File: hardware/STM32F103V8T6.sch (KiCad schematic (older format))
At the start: 34 parts, among them J14 STM32_USB_DEBUG, J15 STM32_GTR, J16 SPI_DEBUG, J17 SWD, SW2 RST, U6 STM32F407VET6, Y3 O_8M

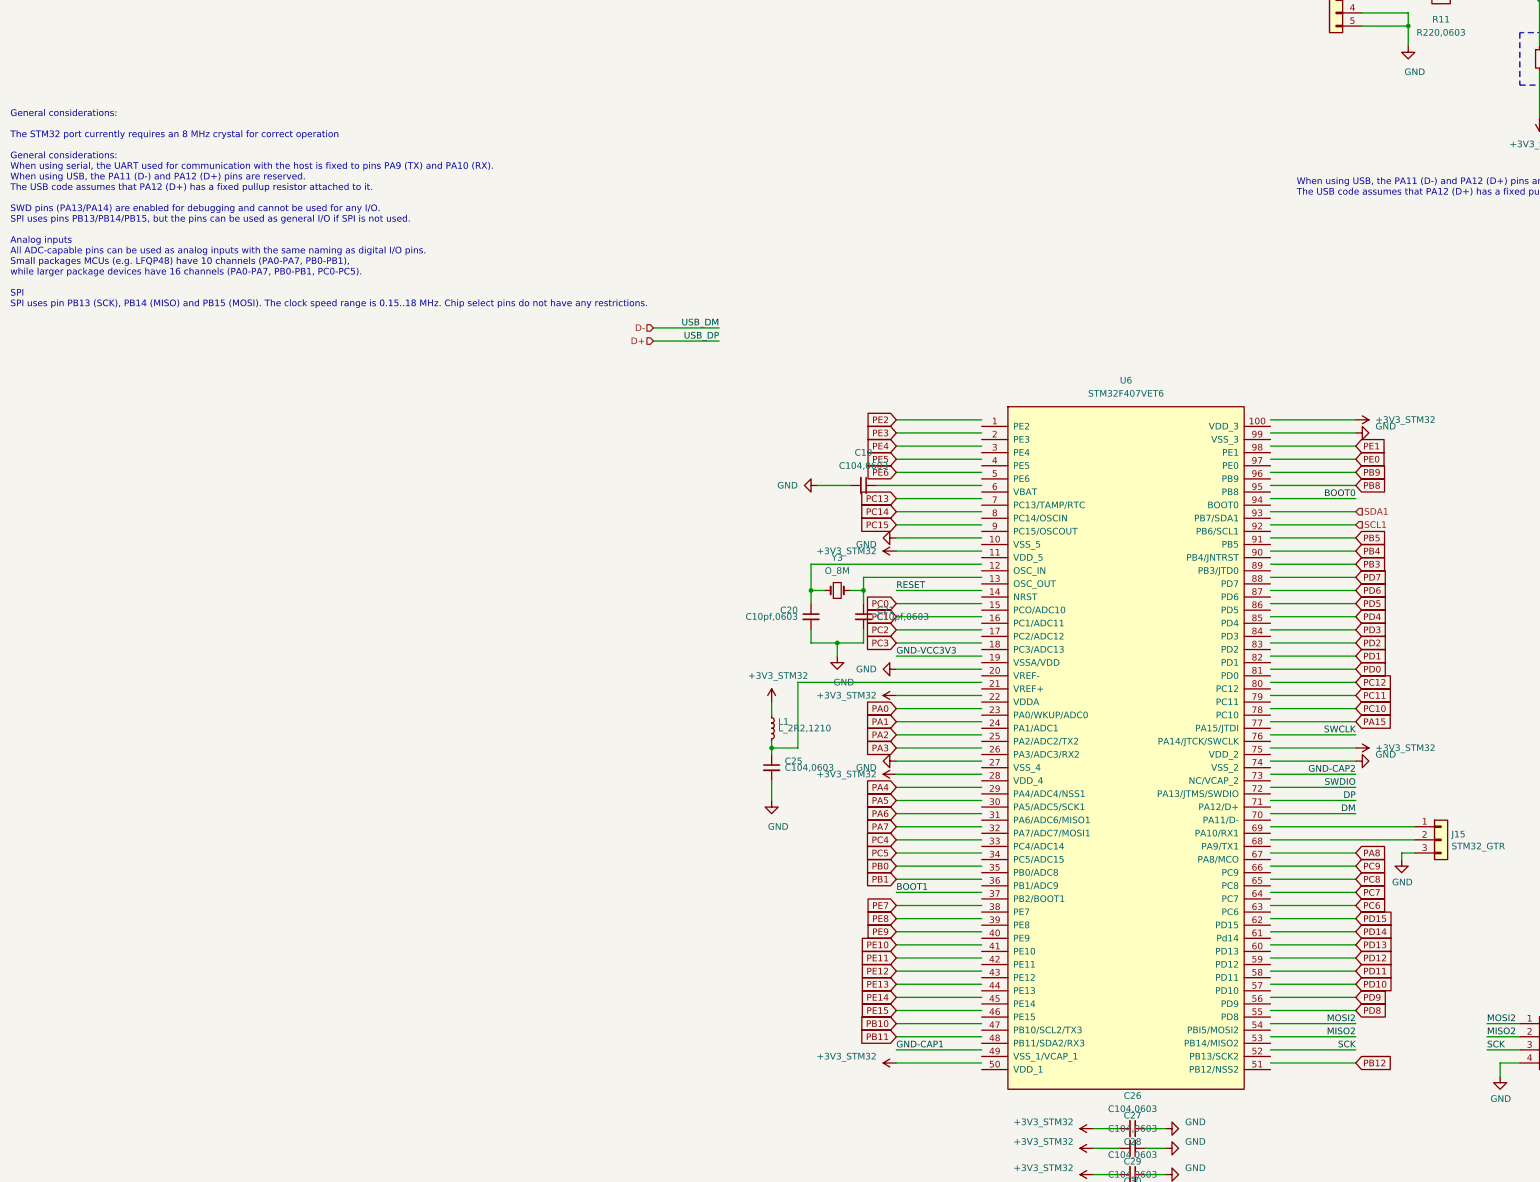
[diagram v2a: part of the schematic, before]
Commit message: update,
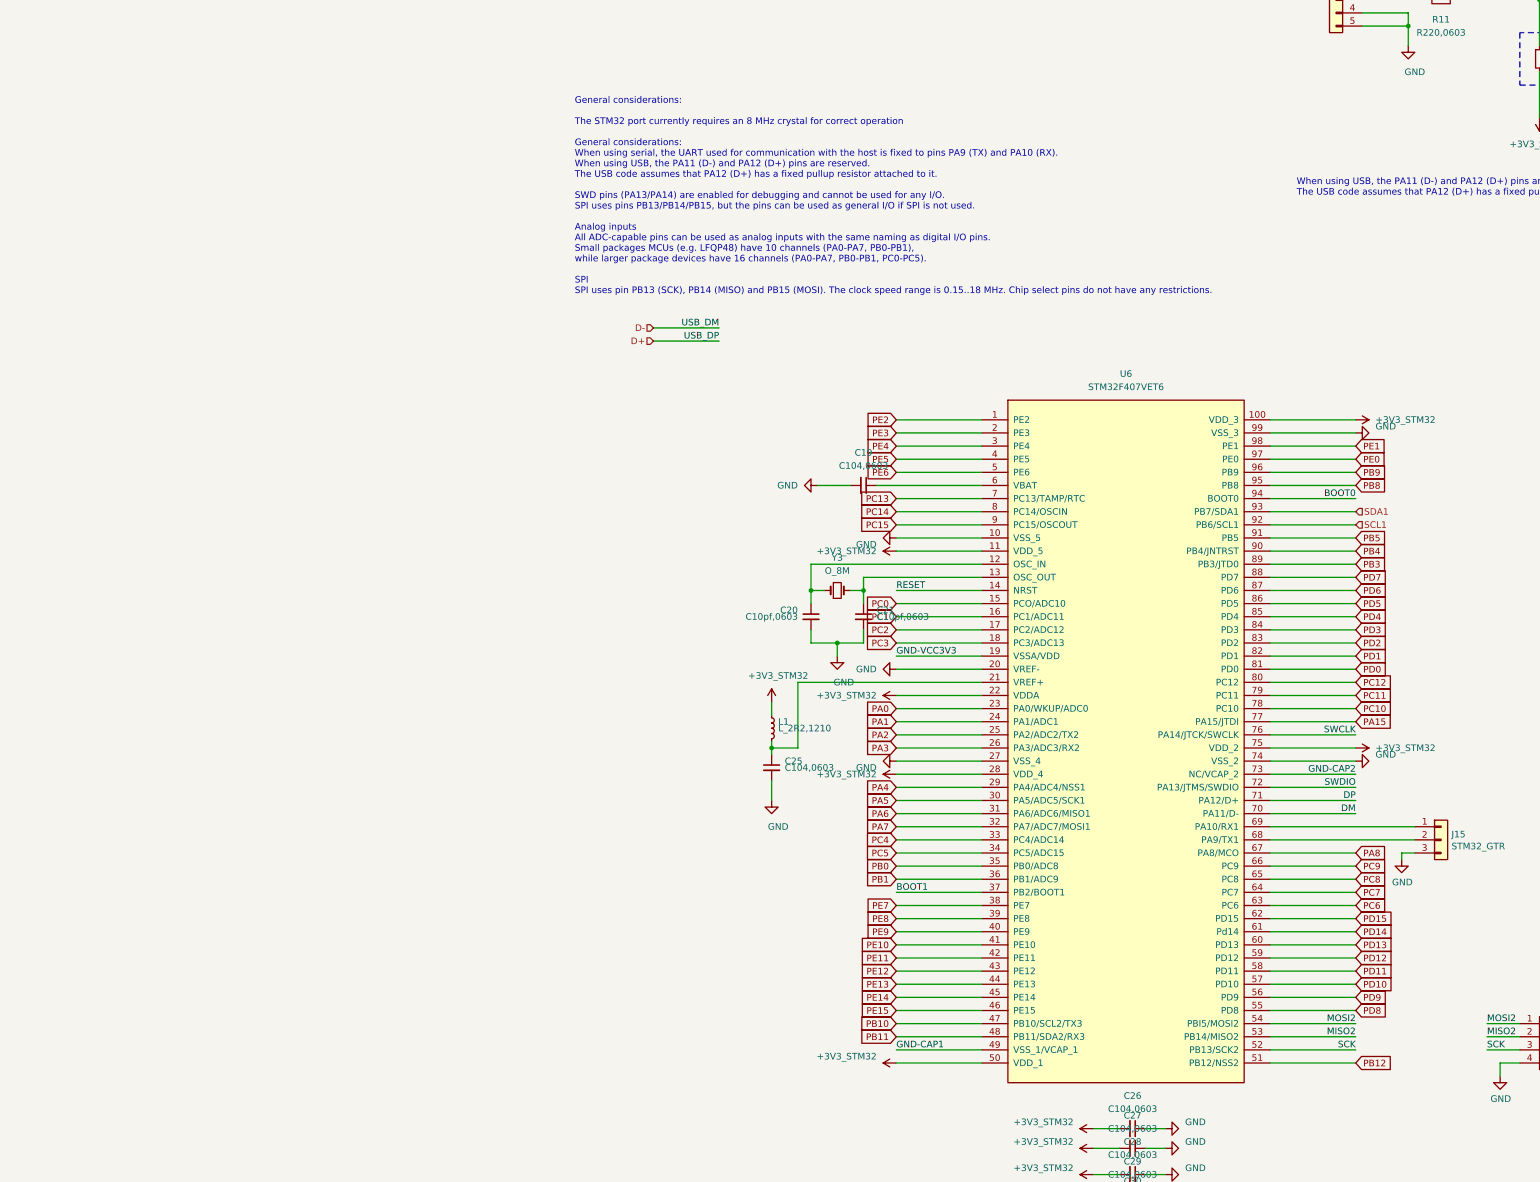
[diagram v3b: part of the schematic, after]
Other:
- moved on the sheet: U6
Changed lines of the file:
@@
 $Descr A3 16535 11693
 encoding utf-8
-Sheet 19 27
+Sheet 24 27
 Title ""
 Date ""
@@
 L taobao-components:STM32F407VET6 U6
 U 1 1 5CC3473C
-P 5000 7000
+P 5000 6950
 AR Path="/5CE045BC/5CC3473C" Ref="U6"  Part="1"
 AR Path="/5CE535D6/5CC3473C" Ref="U?"  Part="1"
-F 0 "U6" H 5000 9750 50  0000 C CNN
-F 1 "STM32F407VET6" H 5000 9650 50  0000 C CNN
-F 2 "w_smd_lqfp:TQFP-100" H 5600 4550 50  0001 C CNN
-F 3 "" H 5600 4550 50  0001 C CNN
-	1    5000 7000
+F 0 "U6" H 5000 9700 50  0000 C CNN
+F 1 "STM32F407VET6" H 5000 9600 50  0000 C CNN
+F 2 "w_smd_lqfp:TQFP-100" H 5600 4500 50  0001 C CNN
+F 3 "" H 5600 4500 50  0001 C CNN
+	1    5000 6950
 	1    0    0    -1
 $EndComp
@@
 Text Label 1900 3950 2    50   ~ 0
 USB_DP
-Text Notes -3500 3700 0    50   ~ 0
+Text Notes 800  3600 0    50   ~ 0
 General considerations:\n\nThe STM32 port currently requires an 8 MHz crystal for correct operation\n\nGeneral considerations:\nWhen using serial, the UART used for communication with the host is fixed to pins PA9 (TX) and PA10 (RX). \nWhen using USB, the PA11 (D-) and PA12 (D+) pins are reserved. \nThe USB code assumes that PA12 (D+) has a fixed pullup resistor attached to it.\n\nSWD pins (PA13/PA14) are enabled for debugging and cannot be used for any I/O. \nSPI uses pins PB13/PB14/PB15, but the pins can be used as general I/O if SPI is not used.\n\nAnalog inputs\nAll ADC-capable pins can be used as analog inputs with the same naming as digital I/O pins. \nSmall packages MCUs (e.g. LFQP48) have 10 channels (PA0-PA7, PB0-PB1), \nwhile larger package devices have 16 channels (PA0-PA7, PB0-PB1, PC0-PC5).\n\nSPI\nSPI uses pin PB13 (SCK), PB14 (MISO) and PB15 (MOSI). The clock speed range is 0.15..18 MHz. Chip select pins do not have any restrictions.
 $Comp
